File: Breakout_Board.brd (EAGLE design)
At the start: 100 x 80 mm, 93 parts, among them IC101 AD8620R, IC102 AD8620R, IC103 ADE7880, IC104 RH/H6, IC105 7805TV, Q101 16M384, U101 ADR512ARTZ-REEL7, U102 SI8640BD-B-IS, U103 SI8641BD-B-IS, X1 231-538/001-000, X101 STL266-04, X103 MKDSN1,5/2-5,08

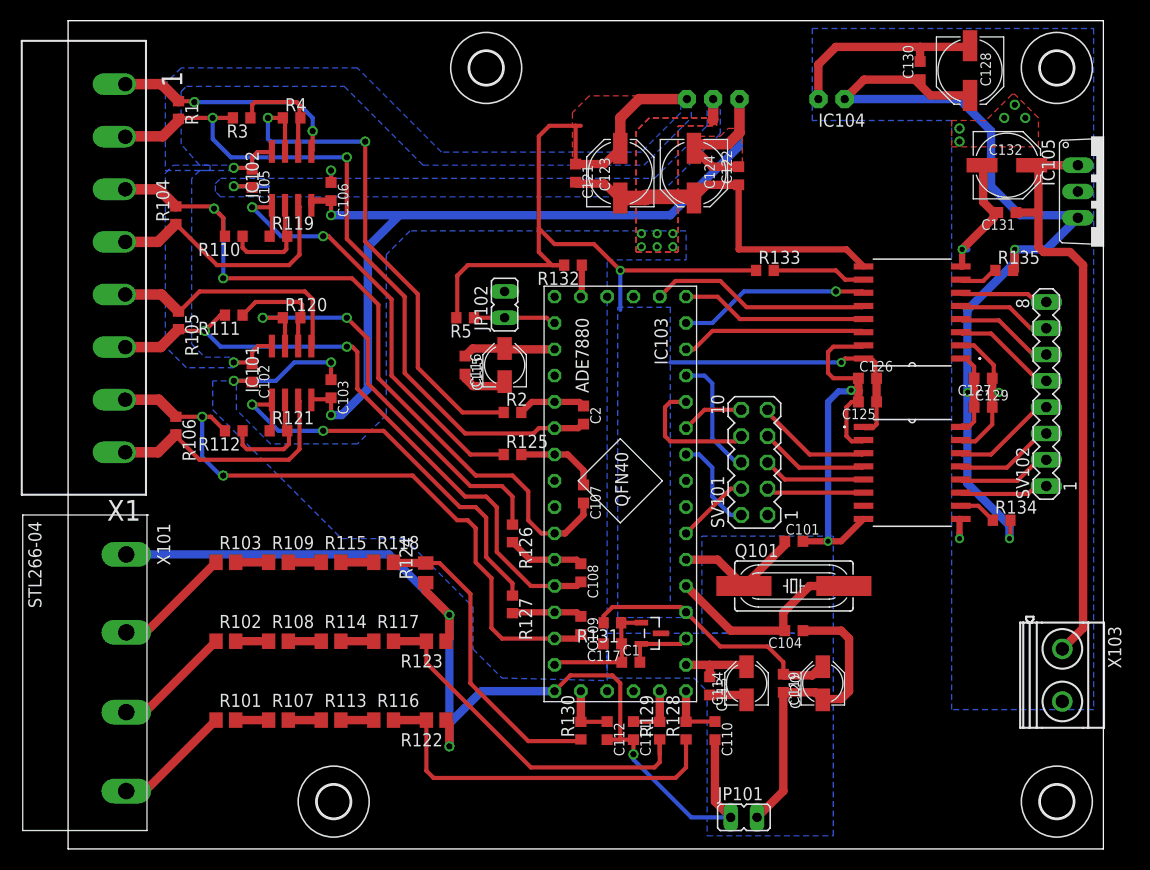
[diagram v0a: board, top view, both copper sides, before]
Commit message: A1 schematic and layout
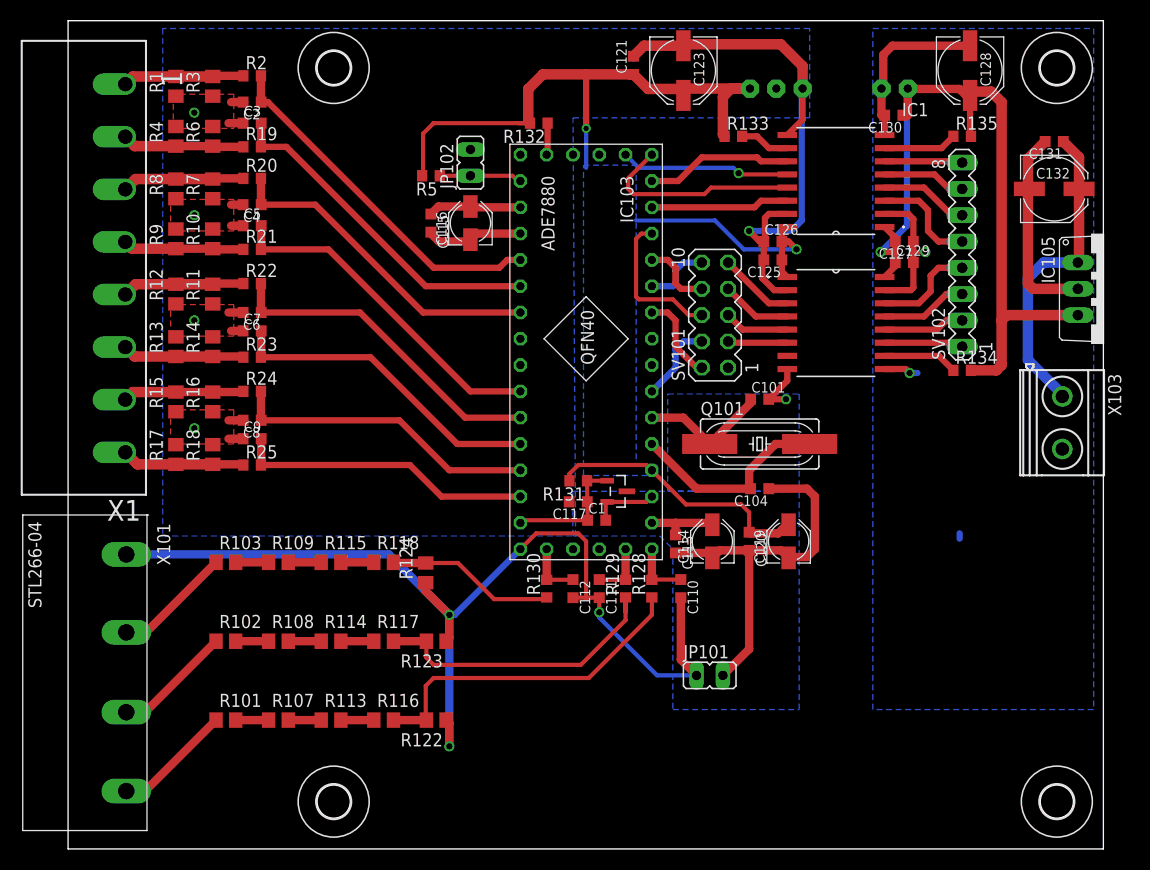
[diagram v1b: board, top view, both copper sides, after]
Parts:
- removed C102, C103, C105, C106: 220n, rcl:C0603K
- removed C107, C108, C109: 2n2, rcl:C0603K
- removed C122: (no value), rcl:C0603K
- removed C124: 47u, rcl:PANASONIC_D
- removed IC101, IC102: AD8620R, analog-devices:SO8
- removed IC104: RH/H6, recom_own:RH/H6
- removed R104, R105, R106: 4R7, rcl:R0603
- removed R110, R111, R112: 6k49, rcl:R0603
- removed R119, R120, R121: 2k21, rcl:R0603
- removed R125, R126, R127: 1k, rcl:R0603
- added C3, C4, C5, C6, C7, C8, C9: 2n2, rcl:C0603K
- added IC1: RH-0505S/H6, recom_own:RH/H6
- added R10, R11, R14, R15, R18, R6, R7: 2R7, rcl:R0805
- added R12, R13, R16, R17, R8, R9: 150R, rcl:R0805
- added R19, R20, R21, R22, R23, R24, R25: 1k, rcl:R0603
- R1: value 4R7 -> 2R7; device rcl:R0603 -> rcl:R0805
- R3: value 6k49 -> 150R; device rcl:R0603 -> rcl:R0805
- R4: value 2k21 -> 150R; device rcl:R0603 -> rcl:R0805
- moved C2 44.0 mm to (17.8, 72.1), turned to 180 degrees
- moved R2 41.1 mm to (17.8, 74.7)
- moved X103 24.4 mm to (96.0, 41.1)
- moved C125 16.5 mm to (68.1, 56.9)
- moved U102 16.2 mm to (74.2, 50.8)
- moved C126 16.1 mm to (68.1, 58.7)
- moved C129 15.9 mm to (80.8, 56.6)
- moved SV102 15.7 mm to (86.4, 57.4)
- moved C127 15.2 mm to (80.8, 58.7)
- moved R134 15.0 mm to (86.4, 46.2)
- moved U$3 14.7 mm to (25.7, 75.4)
- moved SV101 14.7 mm to (62.5, 51.6)
- moved U103 14.7 mm to (74.2, 64.5)
- moved C1 14.1 mm to (51.1, 31.8)
- moved C110 14.1 mm to (59.2, 25.1)
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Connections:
- removed net AGND: C113.2, C114.-
- removed net DGND: C115.2, C116.-
- removed net IN_I1: IC102.3, R104.1, X1.L4
- removed net IN_I2: IC101.5, R105.1, X1.L5
- removed net IN_I3: IC101.3, R106.2, X1.L8
- removed net N$16: IC101.7, R120.1, R126.1
- removed net N$17: IC102.6, R3.1, R4.2
- removed net N$18: IC101.1, R121.1, R127.1
- removed net N$19: IC102.2, R110.1, R119.2
- removed net N$21: IC102.1, R119.1, R125.1
- removed net N$22: IC102.7, R2.1, R4.1
- removed net N$23: IC102.5, R1.1, X1.L1
- removed net N$24: IC101.6, R111.1, R120.2
- removed net N$29: IC101.2, R112.1, R121.2
- removed net VEE: C103.2, C106.2, C122.2, C124.-, IC101.4, IC102.4, IC104.P$3
- new net INH: R15.2, R16.2, R24.1, X1.L7
- new net INL: R17.1, R18.1, R25.1, X1.L8
- new net L1H: R1.2, R2.1, R3.2, X1.L1
- new net L1L: R19.1, R4.1, R6.1, X1.L2
- new net L2H: R20.1, R7.2, R8.2, X1.L3
- new net L2L: R10.1, R21.1, R9.1, X1.L4
- new net L3H: R11.2, R12.2, R22.1, X1.L5
- new net L3L: R13.1, R14.1, R23.1, X1.L6
- net GND: now also C113.2, C114.-, C115.2, C116.-, C2.2, C3.1, C4.2, C5.1, C6.2, C7.1, C8.2, C9.1, IC1.P$3, R1.1, R10.2, R11.1, R12.1, R13.2, R14.2, R15.1, R16.1, R17.2, R18.2, R3.1, R4.2, R6.2, R7.1, R8.1, R9.2; no longer C102.2, C103.1, C105.2, C106.1, C122.1, C124.+, IC104.P$4
- net GND_P: now also IC1.P$2; no longer IC104.P$2
- net IAN: now also C3.2, R19.2; no longer C2.2, R1.2, R3.2, X1.L2
- net IBN: now also C5.2, R21.2; no longer C107.2, R104.2, R110.2, X1.L3
- net IBP: now also C4.1, R20.2; no longer C107.1, R125.2
- net ICN: now also C7.2, R23.2; no longer C108.2, R105.2, R111.2, X1.L6
- net ICP: now also C6.1, R22.2; no longer C108.1, R126.2
- net INN: now also C9.2, R25.2; no longer C109.2, R106.1, R112.2, X1.L7
- net INP: now also C8.1, R24.2; no longer C109.1, R127.2
- net VCC: now also IC1.P$5; no longer C102.1, C105.1, IC101.8, IC102.8, IC104.P$5
- net VCC_P: now also IC1.P$1; no longer IC104.P$1
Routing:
- net VEE: track 90.3 -> 0.00 mm, vias 2 -> 0
- net N$22: track 50.3 -> 0.00 mm, vias 2 -> 0
- net N$21: track 43.7 -> 0.00 mm, vias 2 -> 0
- net N$16: track 41.3 -> 0.00 mm, vias 2 -> 0
- net N$18: track 40.9 -> 0.00 mm, vias 2 -> 0
- net IBN: track 72.2 -> 33.0 mm, vias 2 -> 0
- net IAN: track 70.2 -> 32.9 mm, vias 2 -> 0
- net VCC: track 144.4 -> 108.6 mm, vias 4 -> 2
- net INN: track 63.5 -> 28.9 mm, vias 2 -> 0
- net ICN: track 62.3 -> 31.1 mm, vias 2 -> 0
- net IAP: track 6.59 -> 34.5 mm
- net N$46: track 57.5 -> 30.6 mm
- net ICP: track 7.47 -> 32.0 mm
- net IN_I2: track 24.5 -> 0.00 mm
- net IN_I1: track 24.4 -> 0.00 mm
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- removed copper zone on layer 1, net GND_P
- removed copper zone on layer 1, net VCC
- removed copper zone on layer 1, net VEE
